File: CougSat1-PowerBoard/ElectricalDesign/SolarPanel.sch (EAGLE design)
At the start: 108 parts, among them J1 Wire Harness Connector, U1 SPV1040, U2 SPV1040, U3 TCA9535R, U4 LTC2499, U5 LTC2499, U6 MCP1501-18

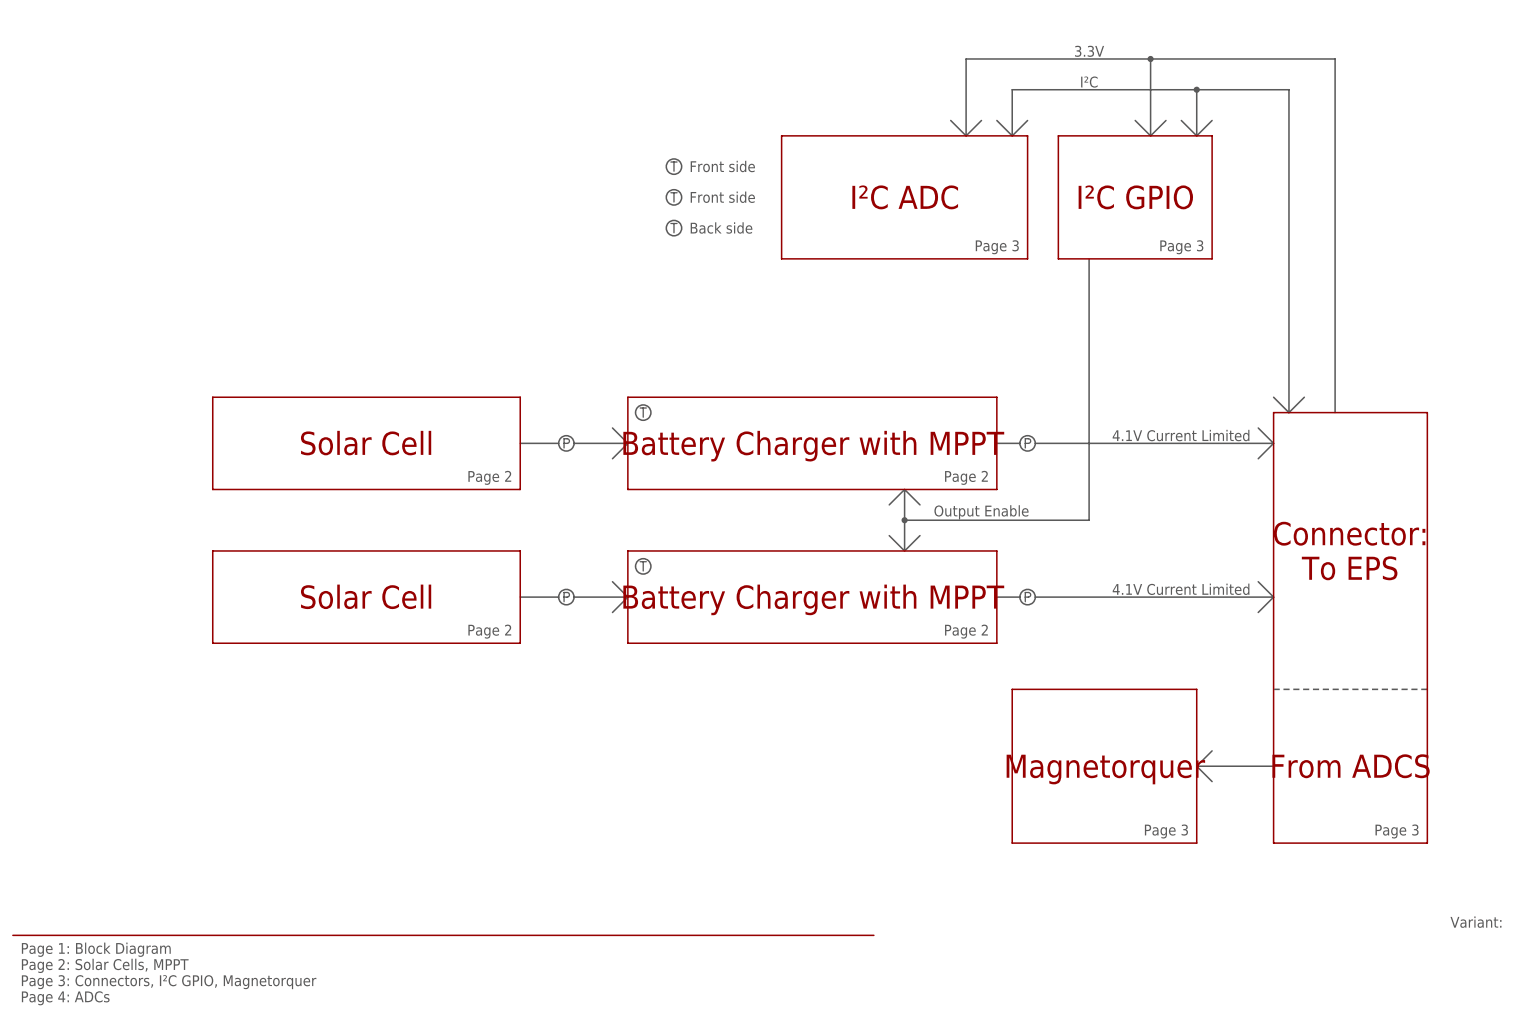
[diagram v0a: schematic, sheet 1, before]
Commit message: Updated Block Diagram
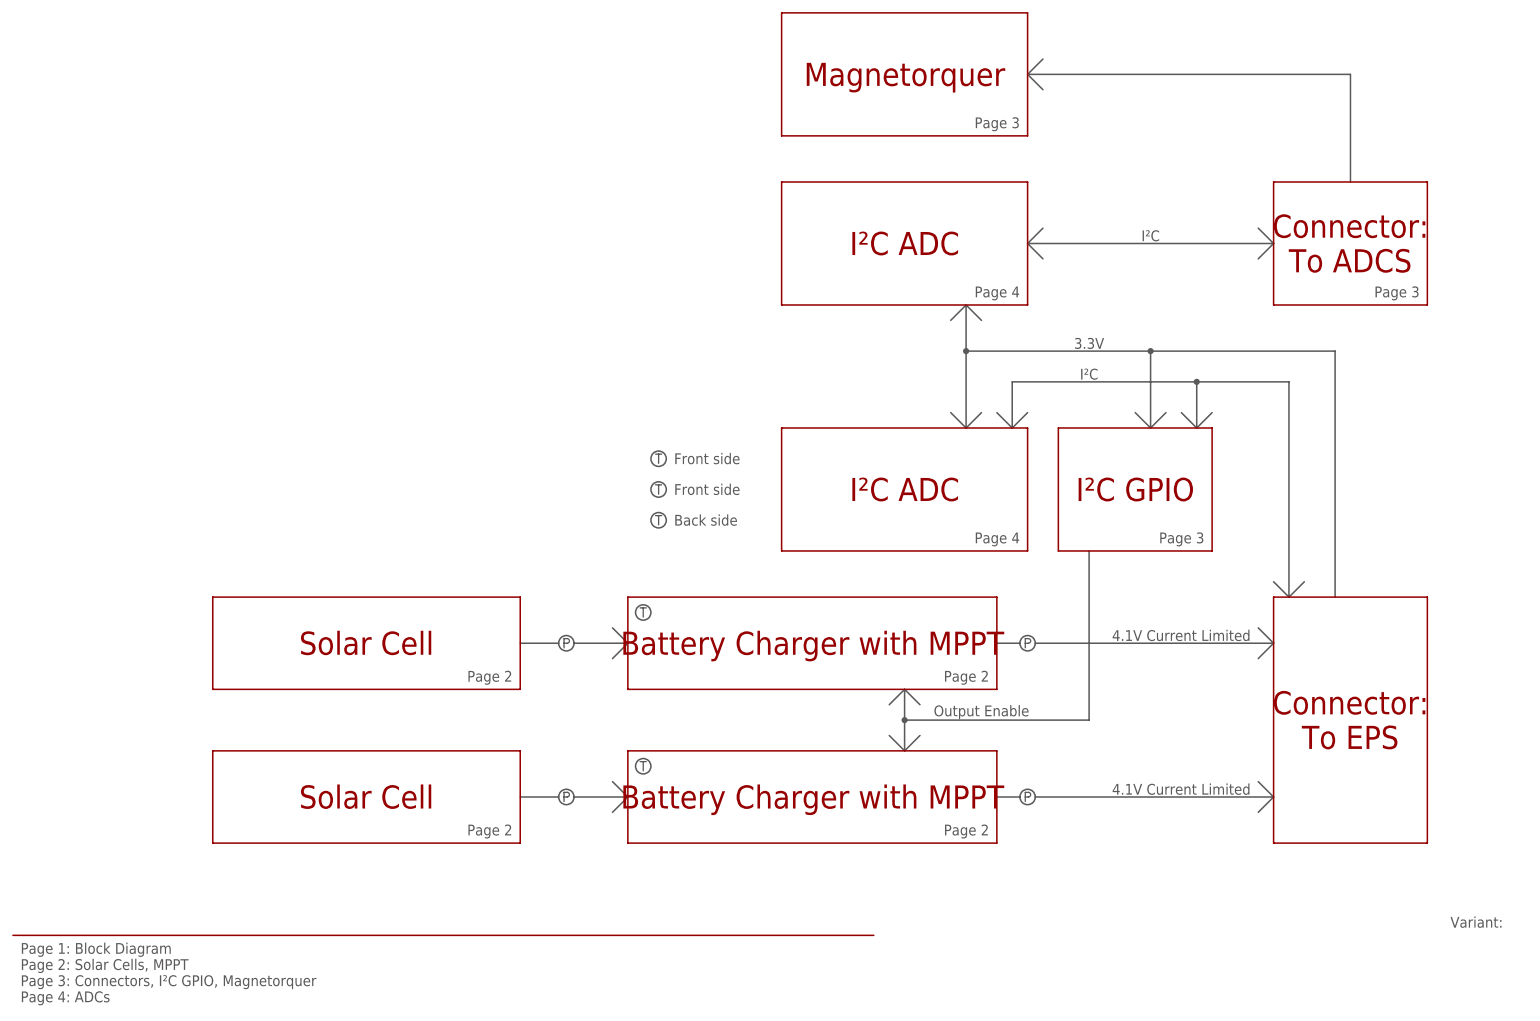
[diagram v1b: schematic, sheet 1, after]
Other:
- note added: "Connector: To ADCS"
- note added: "Page 4"
- note removed: "From ADCS"
